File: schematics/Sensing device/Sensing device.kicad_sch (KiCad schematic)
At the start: 9 parts, among them J1 JST-PH connector, J2 Grove GSR Sensor Module, SW1 SW_DPST, U1 XIAO ESP32-C3

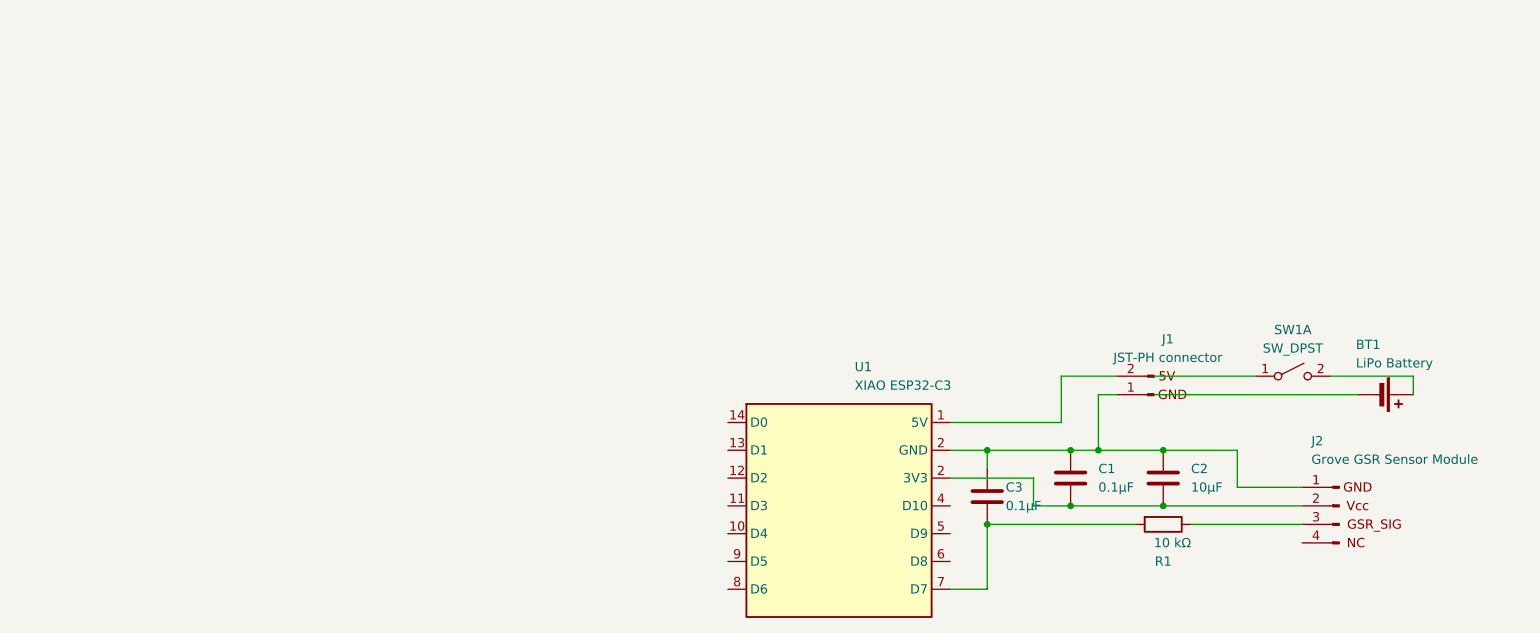
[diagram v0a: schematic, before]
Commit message: device
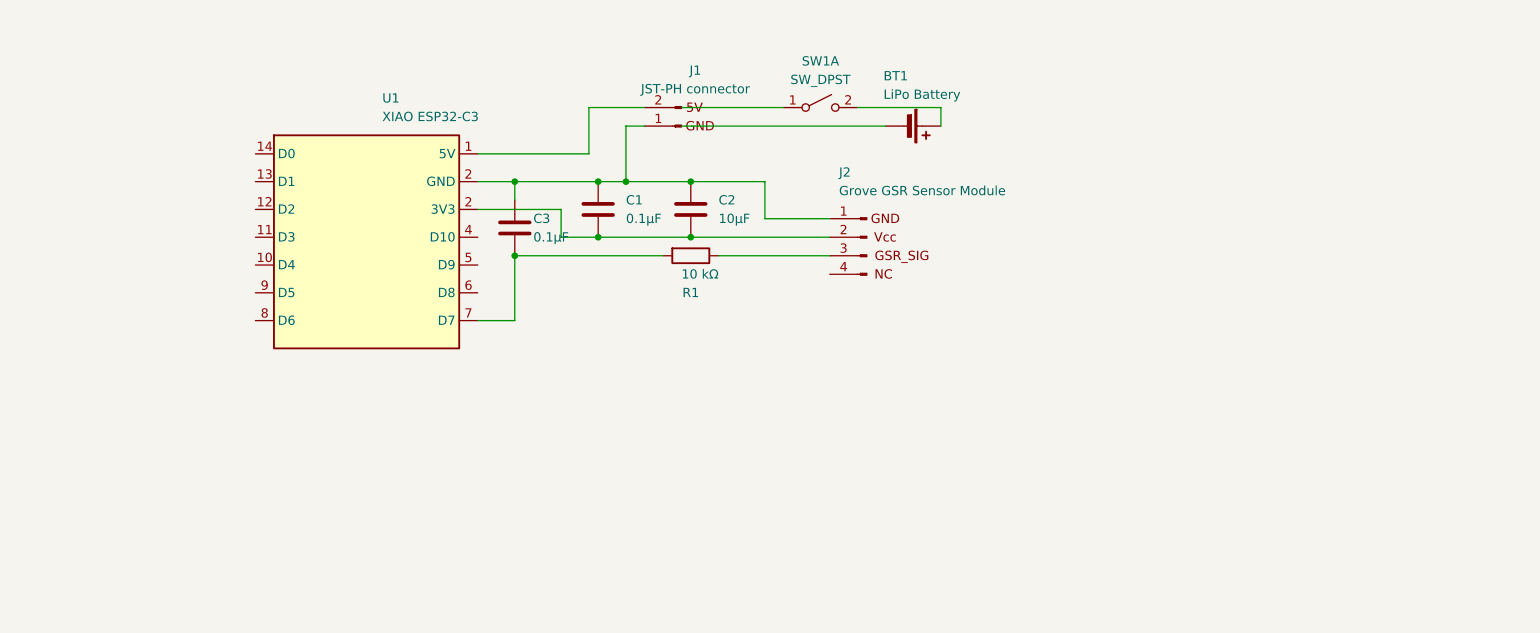
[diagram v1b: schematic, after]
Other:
- moved on the sheet: BT1, C1, C2, C3, J1, J2, R1, SW1A, U1

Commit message: kicad update
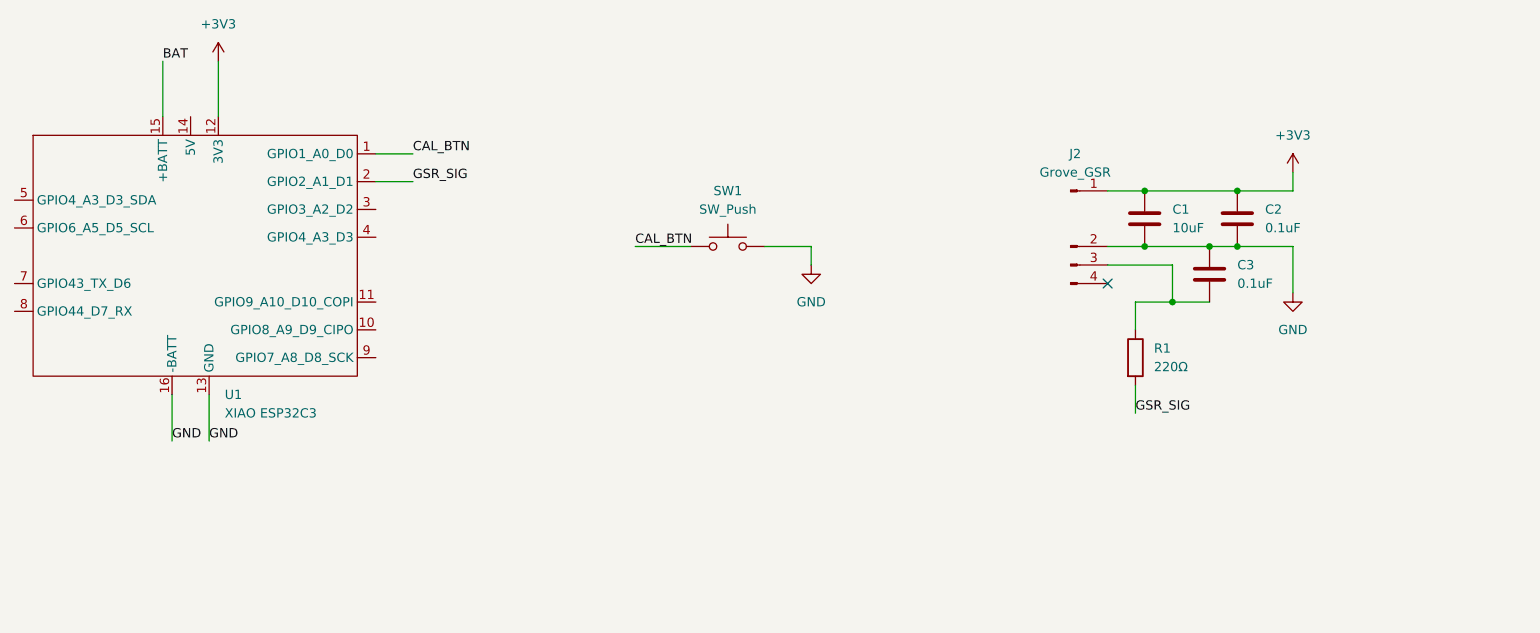
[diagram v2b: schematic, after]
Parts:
- removed BT1: LiPo Battery, symbol Device:Battery_Cell
- removed J1: JST-PH connector, symbol Connector:Conn_01x02_Pin
- removed SW1: SW_DPST, symbol Switch:SW_DPST_x2
- removed U1: XIAO ESP32-C3, RF_Module:ESP32-C3-DevKitM-1, symbol RF_Module:ESP32-C3-DevKitM-1
- added SW1: SW_Push, Button_Switch_SMD:SW_Push_1P1T_NO_E-Switch_TL3301NxxxxxG, symbol Switch:SW_Push
- added U1: XIAO ESP32C3, GIX_ESP32:XIAO_ESP32, symbol GIX_ESP32:XIAO_ESP32
- C1: value 0.1µF -> 10uF; footprint (none) -> Capacitor_SMD:C_0805_2012Metric_Pad1.18x1.45mm_HandSolder
- C2: value 10µF -> 0.1uF; footprint (none) -> Capacitor_SMD:C_0805_2012Metric_Pad1.18x1.45mm_HandSolder
- C3: value 0.1µF -> 0.1uF; footprint (none) -> Capacitor_SMD:C_0805_2012Metric_Pad1.18x1.45mm_HandSolder
- J2: value Grove GSR Sensor Module -> Grove_GSR; footprint (none) -> Connector_JST:JST_PH_S4B-PH-SM4-TB_1x04-1MP_P2.00mm_Horizontal
- R1: value 10 kΩ -> 220Ω; footprint (none) -> Resistor_SMD:R_0805_2012Metric_Pad1.20x1.40mm_HandSolder
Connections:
- net +3V3: now reaches C1.1, C2.1, J2.1 (Pin_1)
- net +3V3: now also U1.12 (3V3); no longer C3.1
- net GND: now reaches C1.2, C2.2, J2.2 (Pin_2)
- net GND: now also C3.1, SW1.2, U1.13 (GND), U1.16 (-BATT)
- net at J2.3 (Pin_3), R1.1: now also C3.2
- net GSR_SIG: now reaches R1.2
- net GSR_SIG: now also U1.2 (GPIO2_A1_D1); no longer C3.2
- new net BAT: U1.15 (+BATT)
- new net CAL_BTN: SW1.1, U1.1 (GPIO1_A0_D0)
- no-connect marks 0 -> 1
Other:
- title: Sensing Device -> Polly Yao_EmoTrace_Sensing Device
